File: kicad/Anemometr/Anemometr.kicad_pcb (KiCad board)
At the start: 2 copper layers, 44.9 x 45.2 mm, 177 parts, among them J1 +5.5v, J10 +Z3, J11 -Z3, J12 +Z4, J13 -Z4, J14 SWD, J15 SWC, J16 Z4, J17 Z4, J18 1 TxD+, J19 2 TxD-, J2 Conn_01x01_Female, J20 3 RxD+, J21 4, J22 5, J23 6 RxD-, J24 7, J25 8, J26 Z4, J27 Z4, J28 Z4, J29 Z4, J3 RST, J30 Z4, J31 Z4, J32 Z4, J33 Z4, J34 Z4, J35 Z4, J36 TMP117, J37 TMP117, J38 TMP117, J39 TMP117, J4 TxD, J5 RxD, J6 +Z1, J7 -Z1, J8 +Z2, J9 -Z2, Q1 5N10, U1 TS5A3166DBVR, U10 MCP1700-3002E, U2 LMV7239, U3 TS5A3166DBVR, U4 TS5A3166DBVR, U5 STM32F103C8Tx, U6 TS5A3166DBVR, U7 LM2734Y, U8 MCP1700-5002E, U9 MCP1700-3002E, Y1 8MHz, Y2 25MHz

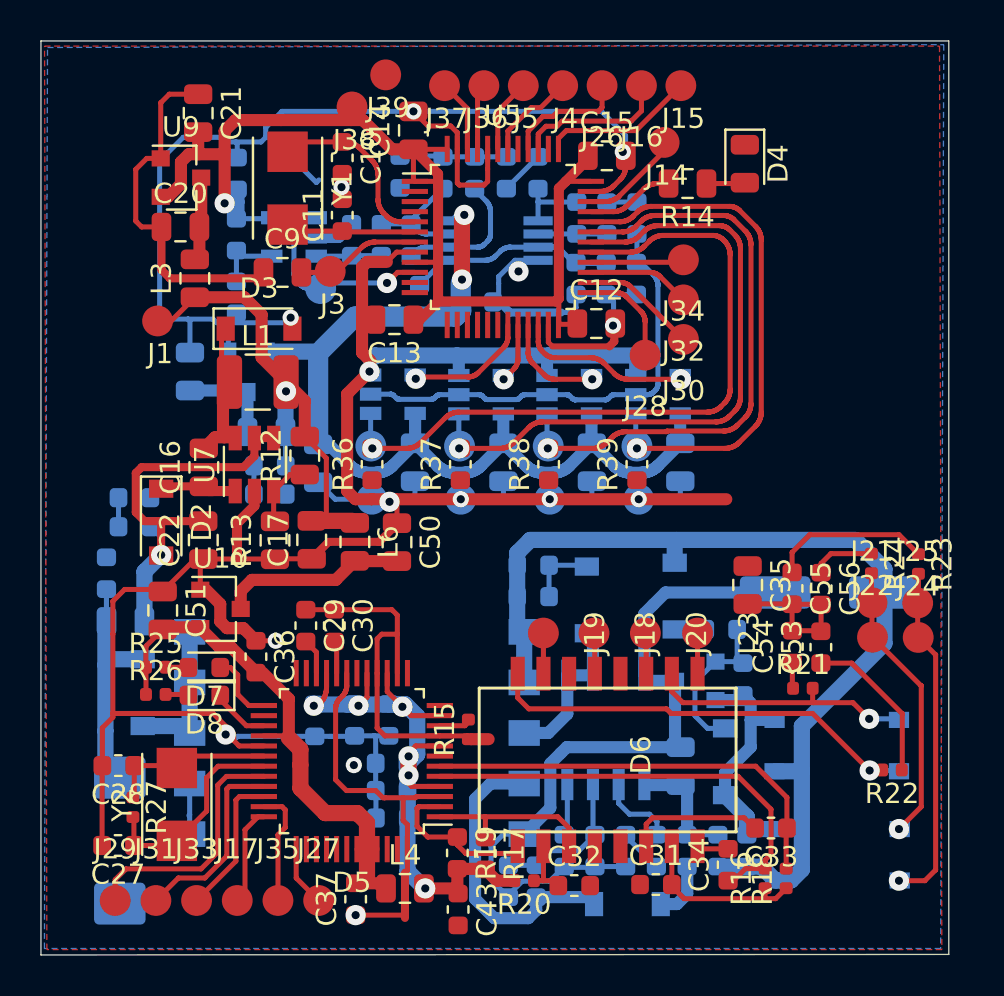
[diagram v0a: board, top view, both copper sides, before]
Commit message: изменено:      kicad/Anemometr/Anemometr.kicad_pcb 	изменено:      kicad/Anemometr/Anemometr.kicad_pcb-bak 	изменено:      kicad/Anemometr/Anemometr.sch 	изменено:      kicad/Anemometr/Anemometr.sch-bak 	изменено:      kicad/Anemometr/fp-info-cache 	изменено:      stm32cubeide/Anemometer/.cproject 	изменено:      stm32cubeide/Anemometer/.mxproject 	изменено:      stm32cubeide/Anemometer/.project 	изменено:      stm32cubeide/Anemometer/Anemometer.ioc 	изменено:      stm32cubeide/Anemometer/Core/Inc/main.h 	изменено:      stm32cubeide/Anemometer/Core/Inc/stm32f1xx_hal_conf.h 	новый файл:    stm32cubeide/Anemometer/Core/Inc/w5500.h 	новый файл:    stm32cubeide/Anemometer/Core/Inc/wizchip_conf.h 	новый файл:    stm32cubeide/Anemometer/Core/Src/dhcp.c 	новый файл:    stm32cubeide/Anemometer/Core/Src/dns.c 	изменено:      stm32cubeide/Anemometer/Core/Src/main.c 	новый файл:    stm32cubeide/Anemometer/Core/Src/socket.c 	изменено:      stm32cubeide/Anemometer/Core/Src/stm32f1xx_hal_msp.c 	новый файл:    stm32cubeide/Anemometer/Core/Src/w5500.c 	новый файл:    stm32cubeide/Anemometer/Core/Src/wizchip_conf.c 	удалено:       stm32cubeide/Anemometer/Drivers/STM32F1xx_HAL_Driver/Inc/stm32f1xx_hal_spi.h 	удалено:       stm32cubeide/Anemometer/Drivers/STM32F1xx_HAL_Driver/Src/stm32f1xx_hal_spi.c 	изменено:      stm32cubeide/Anemometer/Release/Anemometer.bin 	изменено:      stm32cubeide/Anemometer/Release/Anemometer.elf 	изменено:      stm32cubeide/Anemometer/Release/Anemometer.list 	изменено:      stm32cubeide/Anemometer/Release/Anemometer.map 	изменено:      stm32cubeide/Anemometer/Release/Core/Src/main.d 	изменено:      stm32cubeide/Anemometer/Release/Core/Src/main.o 	изменено:      stm32cubeide/Anemometer/Release/Core/Src/main.su 	изменено:      stm32cubeide/Anemometer/Release/Core/Src/stm32f1xx_hal_msp.d 	изменено:      stm32cubeide/Anemometer/Release/Core/Src/stm32f1xx_hal_msp.o 	изменено:      stm32cubeide/Anemometer/Release/Core/Src/stm32f1xx_hal_msp.su 	изменено:      stm3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
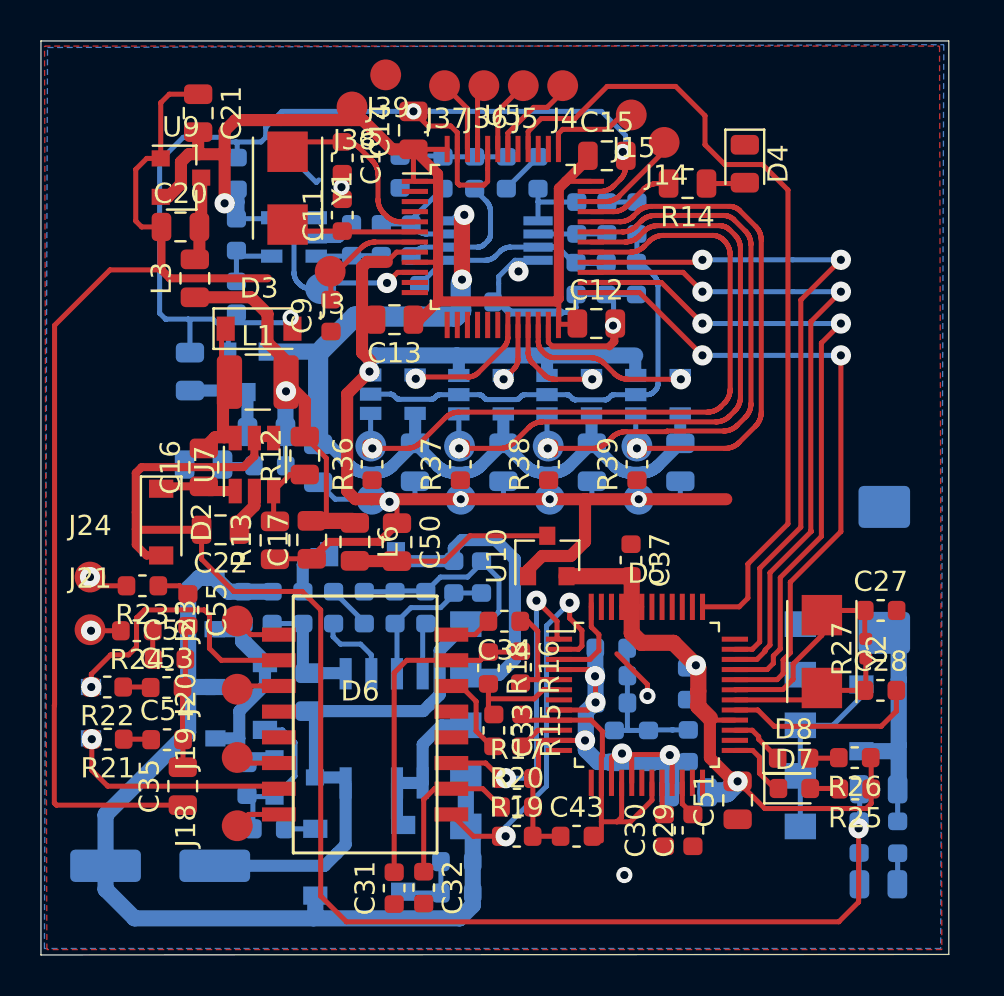
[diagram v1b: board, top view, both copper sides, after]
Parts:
- removed J1: +5.5v, My-library:SMD-CONN
- removed J16, J17, J26, J27, J28, J29, J30, J31, J32, J33, J34, J35: Z4, My-library:SMD-CONN
- removed J22: 5, My-library:SMD-CONN
- removed J25: 8, My-library:SMD-CONN
- C36, L4: moved to B.Cu
- C9: footprint Capacitor_SMD:C_0805_2012Metric -> Capacitor_SMD:C_0603_1608Metric
- D18, D19: footprint LED_SMD:LED_0603_1608Metric -> LED_SMD:LED_0805_2012Metric
- J21: value 4 -> 4-5
- J24: value 7 -> 7-8
- R15, R16, R18, R20, R21, R22, R23, R24, R25, R26: footprint Resistor_SMD:R_0402_1005Metric -> Resistor_SMD:R_0603_1608Metric
- moved D18 41.4 mm to (60.3, 101.3)
- moved R35 41.2 mm to (61.2, 99.0), turned to 270 degrees
- moved J24 41.1 mm to (21.3, 86.1)
- moved C49 40.1 mm to (60.6, 85.8), turned to 90 degrees
- moved C27 39.5 mm to (60.4, 87.8), turned to 0 degrees
- moved R22 39.0 mm to (22.1, 91.5)
- moved R43 39.0 mm to (59.3, 99.0), turned to 90 degrees
- moved J21 38.7 mm to (21.3, 88.7)
- moved R23 38.4 mm to (23.9, 86.5), turned to 180 degrees
- moved L5 38.2 mm to (60.3, 96.6), turned to 0 degrees
- moved C28 37.9 mm to (60.4, 91.7), turned to 0 degrees
- moved R27 37.1 mm to (59.7, 89.6), turned to 90 degrees
- moved R24 36.5 mm to (23.6, 88.8), turned to 180 degrees
- moved D10 36.1 mm to (24.4, 87.4), turned to 0 degrees
- moved C45 35.8 mm to (24.8, 100.4), turned to 0 degrees
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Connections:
- D5 pad 36: Net-(D5-Pad36) -> (no net)
- D9 pad 1: Net-(D6-Pad10) -> Net-(D6-Pad15)
- D9 pad 2: Net-(D6-Pad15) -> Net-(D6-Pad10)
- R21 pad 2: Net-(D6-Pad10) -> Net-(D6-Pad15)
- R22 pad 2: Net-(D6-Pad15) -> Net-(D6-Pad10)
- U5 pad 25: Net-(J28-Pad1) -> Net-(D5-Pad32)
- U5 pad 26: Net-(J30-Pad1) -> Net-(D5-Pad33)
- U5 pad 27: Net-(J32-Pad1) -> Net-(D5-Pad34)
- U5 pad 28: Net-(J34-Pad1) -> Net-(D5-Pad35)
- U5 pad 39: Net-(J16-Pad1) -> (no net)
- U5 pad 40: Net-(J26-Pad1) -> Net-(D5-Pad37)
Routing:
- net Net-(C22-Pad2): track 20.5 -> 71.7 mm
- net Net-(D5-Pad37): track 3.00 -> 41.0 mm
- net Net-(D5-Pad35): track 5.75 -> 34.3 mm, vias 0 -> 2
- net Net-(D5-Pad34): track 7.22 -> 33.8 mm, vias 0 -> 2
- net Net-(D5-Pad33): track 9.62 -> 33.4 mm, vias 0 -> 2
- net Net-(D5-Pad32): track 12.4 -> 33.1 mm, vias 0 -> 2
- net Net-(C34-Pad1): track 22.2 -> 5.43 mm
- net Net-(C33-Pad1): track 21.3 -> 5.30 mm
- net Net-(D10-Pad2): track 17.1 -> 1.98 mm
- net Net-(D10-Pad1): track 14.2 -> 1.54 mm
- net Net-(D5-Pad2): track 7.96 -> 19.3 mm, vias 0 -> 2
- net Net-(D6-Pad15): track 22.2 -> 11.2 mm
- net Net-(C31-Pad2): track 8.63 -> 16.5 mm
- net Net-(J16-Pad1): track 7.57 -> 0.00 mm
- net Net-(D5-Pad1): track 8.56 -> 15.2 mm, vias 0 -> 2
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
